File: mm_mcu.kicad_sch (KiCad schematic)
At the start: 17 parts, among them J1 Conn_ARM_JTAG_SWD_10, U1 STM32F030C8Tx

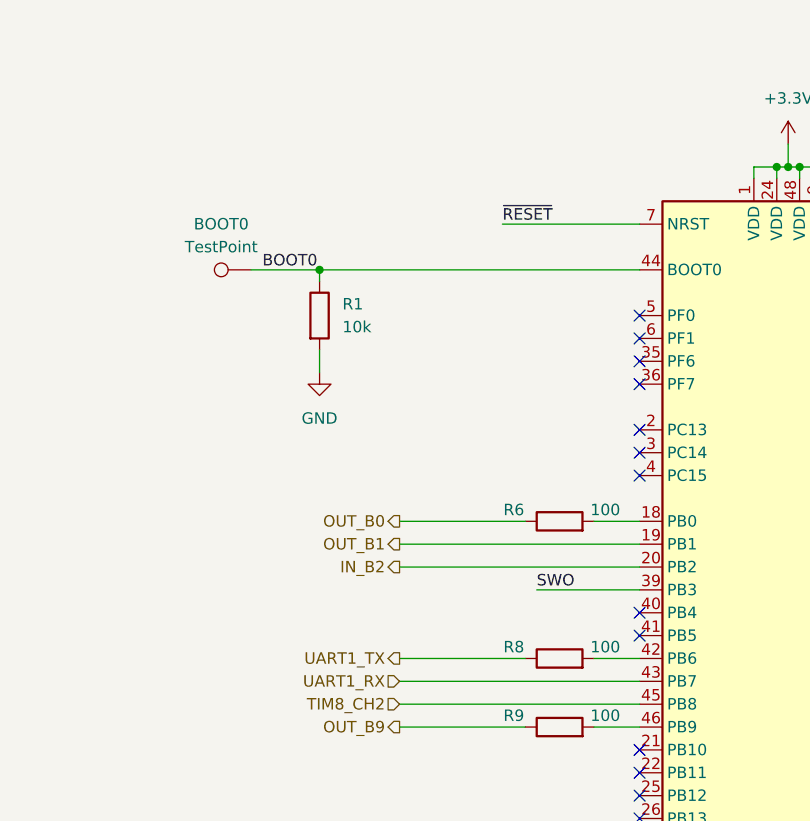
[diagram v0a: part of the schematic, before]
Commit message: tp5
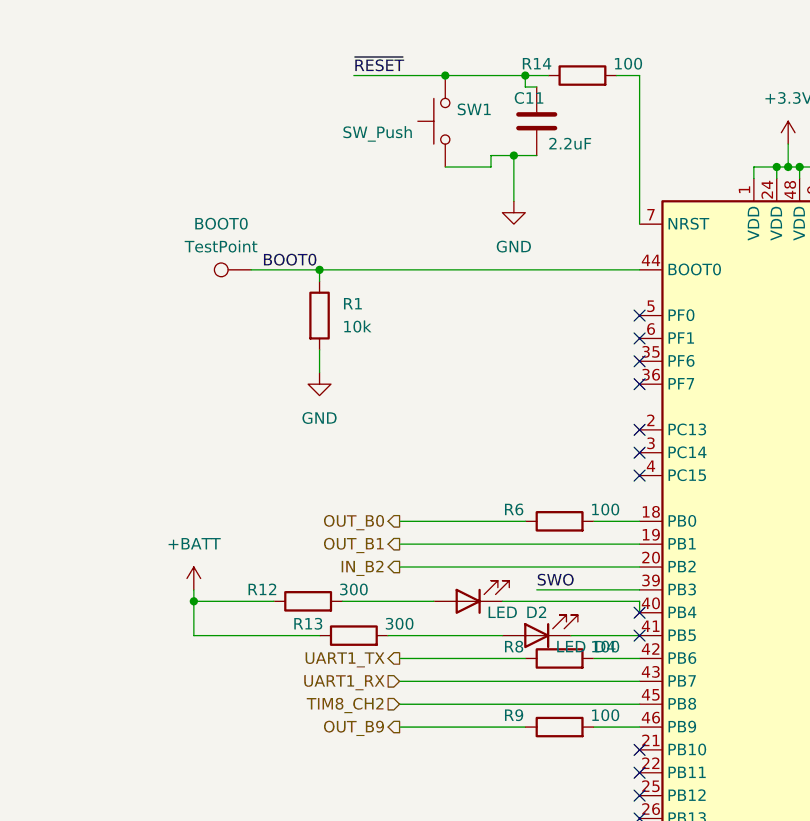
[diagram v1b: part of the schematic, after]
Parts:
- added C11: 2.2uF, Capacitor_SMD:C_0603_1608Metric, symbol Device:C
- added D2, D4: LED, LED_SMD:LED_0603_1608Metric, symbol Device:LED
- added R12, R13: 300, Resistor_SMD:R_0603_1608Metric, symbol Device:R
- added R14: 100, Resistor_SMD:R_0603_1608Metric, symbol Device:R
- added SW1: SW_Push, Button_Switch_SMD:SW_Push_SPST_NO_Alps_SKRK, symbol Switch:SW_Push
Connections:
- net GND: now also C11.2, SW1.1
- net ~{RESET}: now also C11.1, R14.1, SW1.2; no longer U1.7 (NRST)
- net at U1.40 (PB4): now also D2.1 (K)
- net at U1.41 (PB5): now also D4.1 (K)
- new net: D2.2 (A), R12.2
- new net: D4.2 (A), R13.2
- new net: R14.2, U1.7 (NRST)
- new net +BATT: R12.1, R13.1
